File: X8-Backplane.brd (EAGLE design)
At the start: 101.6 x 101.6 mm, 4 parts

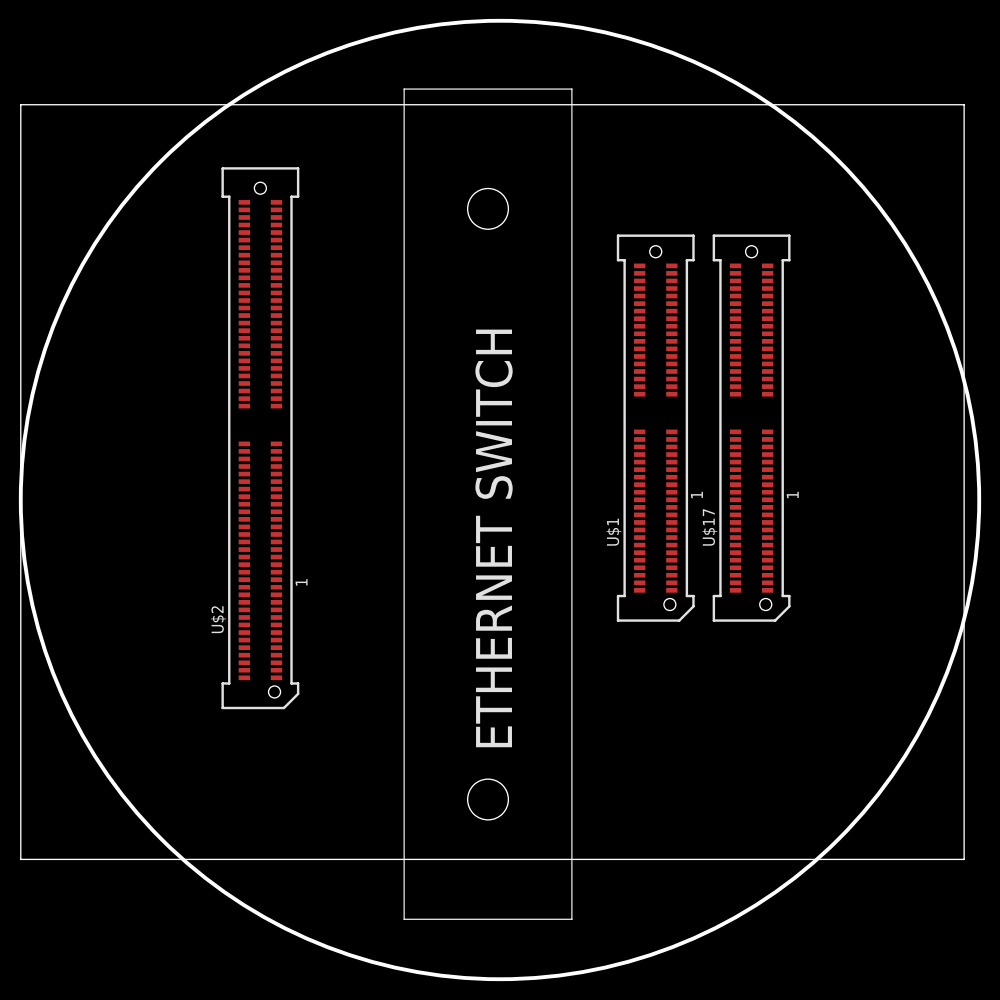
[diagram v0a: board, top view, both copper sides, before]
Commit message: Fleshing out the idea for the backplane
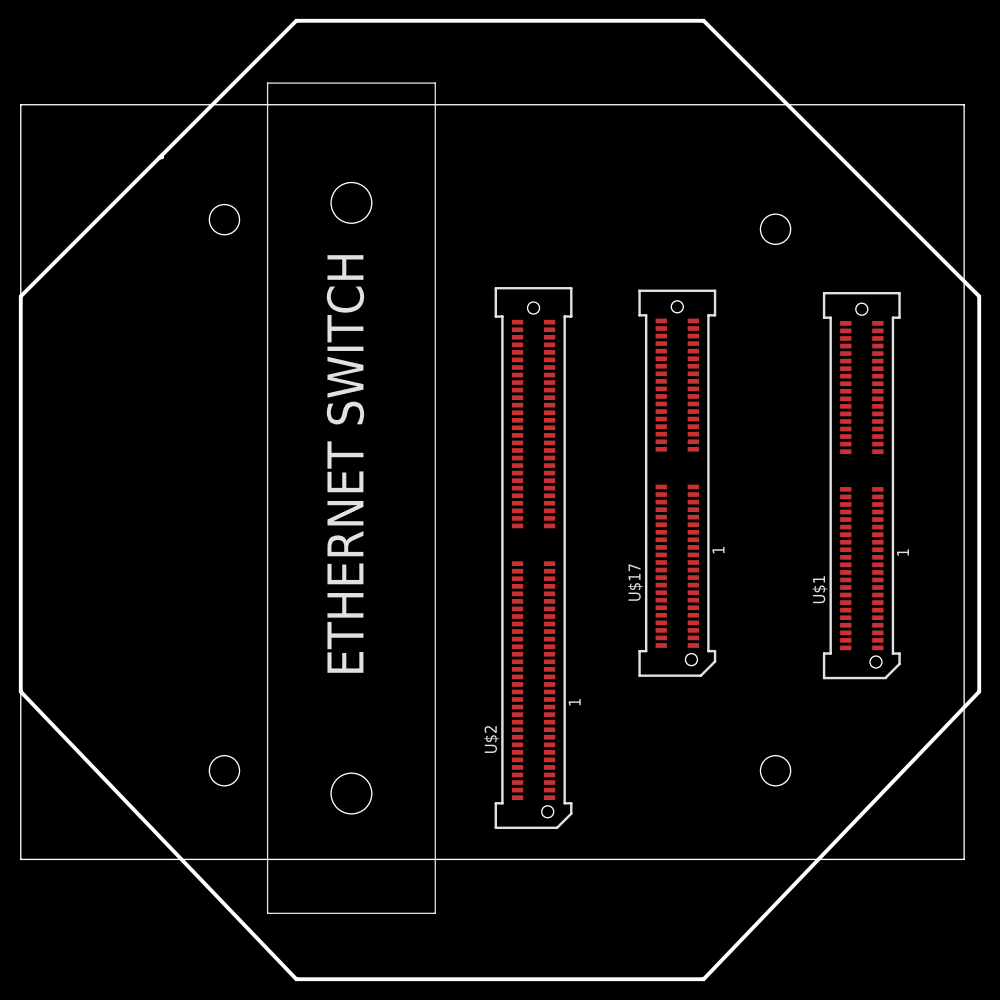
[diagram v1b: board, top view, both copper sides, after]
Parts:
- moved U$18 94.3 mm to (26.2, 82.3), turned to 270 degrees
- moved U$2 31.6 mm to (54.4, 31.8)
- moved U$1 22.7 mm to (89.2, 39.6)
- moved U$17 9.80 mm to (69.6, 39.9)
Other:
- outline, holes or cut-outs redrawn
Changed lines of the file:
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@@
 <setting verticaltext="up"/>
 </settings>
-<grid distance="0.05" unitdist="inch" unit="inch" style="lines" multiple="1" display="no" altdistance="0.025" altunitdist="inch" altunit="inch"/>
+<grid distance="0.01" unitdist="inch" unit="inch" style="lines" multiple="1" display="no" altdistance="0.025" altunitdist="inch" altunit="inch"/>
 <layers>
 <layer number="1" name="Top" color="4" fill="1" visible="yes" active="yes"/>
@@
 <layer number="42" name="bRestrict" color="1" fill="10" visible="no" active="yes"/>
 <layer number="43" name="vRestrict" color="2" fill="10" visible="no" active="yes"/>
-<layer number="44" name="Drills" color="7" fill="1" visible="yes" active="yes"/>
+<layer number="44" name="Drills" color="7" fill="1" visible="no" active="yes"/>
 <layer number="45" name="Holes" color="7" fill="1" visible="yes" active="yes"/>
-<layer number="46" name="Milling" color="3" fill="1" visible="yes" active="yes"/>
-<layer number="47" name="Measures" color="7" fill="1" visible="yes" active="yes"/>
-<layer number="48" name="Document" color="7" fill="1" visible="yes" active="yes"/>
+<layer number="46" name="Milling" color="3" fill="1" visible="no" active="yes"/>
+<layer number="47" name="Measures" color="7" fill="1" visible="no" active="yes"/>
+<layer number="48" name="Document" color="7" fill="1" visible="no" active="yes"/>
 <layer number="49" name="Reference" color="7" fill="1" visible="no" active="yes"/>
 <layer number="50" name="dxf" color="7" fill="1" visible="no" active="no"/>
-<layer number="51" name="tDocu" color="7" fill="1" visible="no" active="yes"/>
-<layer number="52" name="bDocu" color="7" fill="1" visible="no" active="yes"/>
+<layer number="51" name="tDocu" color="7" fill="1" visible="yes" active="yes"/>
+<layer number="52" name="bDocu" color="7" fill="1" visible="yes" active="yes"/>
 <layer number="53" name="tGND_GNDA" color="7" fill="1" visible="no" active="no"/>
 <layer number="54" name="bGND_GNDA" color="7" fill="1" visible="no" active="no"/>
@@
 <wire x1="100" y1="0" x2="100" y2="80" width="0" layer="20"/>
 <wire x1="100" y1="80" x2="0" y2="80" width="0" layer="20"/>
-<wire x1="0" y1="80" x2="0" y2="0" width="0" layer="20"/>
-<circle x="50.8" y="38.1" radius="50.8" width="0.4064" layer="20"/>
+<wire x1="0" y1="80" x2="0" y2="59.69" width="0" layer="20"/>
+<wire x1="0" y1="17.78" x2="0" y2="0" width="0" layer="20"/>
+<wire x1="0" y1="59.69" x2="0" y2="17.78" width="0.4064" layer="20"/>
+<wire x1="29.21" y1="-12.7" x2="72.39" y2="-12.7" width="0.4064" layer="20"/>
+<wire x1="101.6" y1="17.78" x2="101.6" y2="59.69" width="0.4064" layer="20"/>
+<wire x1="72.39" y1="88.9" x2="29.21" y2="88.9" width="0.4064" layer="20"/>
+<wire x1="0" y1="59.69" x2="14.732" y2="74.422" width="0.4064" layer="20"/>
+<wire x1="14.732" y1="74.422" x2="29.21" y2="88.9" width="0.4064" layer="20"/>
+<wire x1="29.21" y1="-12.7" x2="0" y2="17.78" width="0.4064" layer="20"/>
+<wire x1="101.6" y1="59.69" x2="72.39" y2="88.9" width="0.4064" layer="20"/>
+<wire x1="101.6" y1="17.78" x2="72.39" y2="-12.7" width="0.4064" layer="20"/>
+<hole x="21.59" y="67.818" drill="3.2"/>
+<hole x="80.01" y="66.802" drill="3.2"/>
+<hole x="21.59" y="9.398" drill="3.2"/>
+<hole x="80.01" y="9.398" drill="3.2"/>
+<wire x1="14.986" y1="74.422" x2="14.732" y2="74.422" width="0.4064" layer="20"/>
 </plain>
 <attributes>
@@
 </autorouter>
 <elements>
-<element name="U$1" library="HSEC8-1xx-01-XX-DV-A" package="HSEC8-140-01-XX-DV-A" value="HSEC8-140-01-XX-DV-A" x="67.31" y="45.72" rot="R90"/>
-<element name="U$17" library="HSEC8-1xx-01-XX-DV-A" package="HSEC8-140-01-XX-DV-A" value="HSEC8-140-01-XX-DV-A" x="77.47" y="45.72" rot="R90"/>
-<element name="U$2" library="HSEC8-1xx-01-XX-DV-A" package="HSEC8-160-01-XX-DV-A" value="HSEC8-160-01-XX-DV-A" x="25.4" y="44.45" rot="R90"/>
-<element name="U$18" library="Other" package="ETH_SWITCH" value="" x="58.42" y="-6.35" rot="R90"/>
+<element name="U$1" library="HSEC8-1xx-01-XX-DV-A" package="HSEC8-140-01-XX-DV-A" value="HSEC8-140-01-XX-DV-A" x="89.154" y="39.624" rot="R90"/>
+<element name="U$17" library="HSEC8-1xx-01-XX-DV-A" package="HSEC8-140-01-XX-DV-A" value="HSEC8-140-01-XX-DV-A" x="69.596" y="39.878" rot="R90"/>
+<element name="U$18" library="Other" package="ETH_SWITCH" value="" x="26.162" y="82.296" rot="R270"/>
+<element name="U$2" library="HSEC8-1xx-01-XX-DV-A" package="HSEC8-160-01-XX-DV-A" value="HSEC8-160-01-XX-DV-A" x="54.356" y="31.75" rot="R90"/>
 </elements>
 <signals>
